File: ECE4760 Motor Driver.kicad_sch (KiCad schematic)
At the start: 29 parts, among them J1 IO, J101 Alternative Motor, J2 Motor / Power, J3 UART, SW1 RESET, U1 STM32G473CETx, U13 AP63205WU, U6 AP7361C-33FGE, U9 MAX13433EETD, X1 48MHz

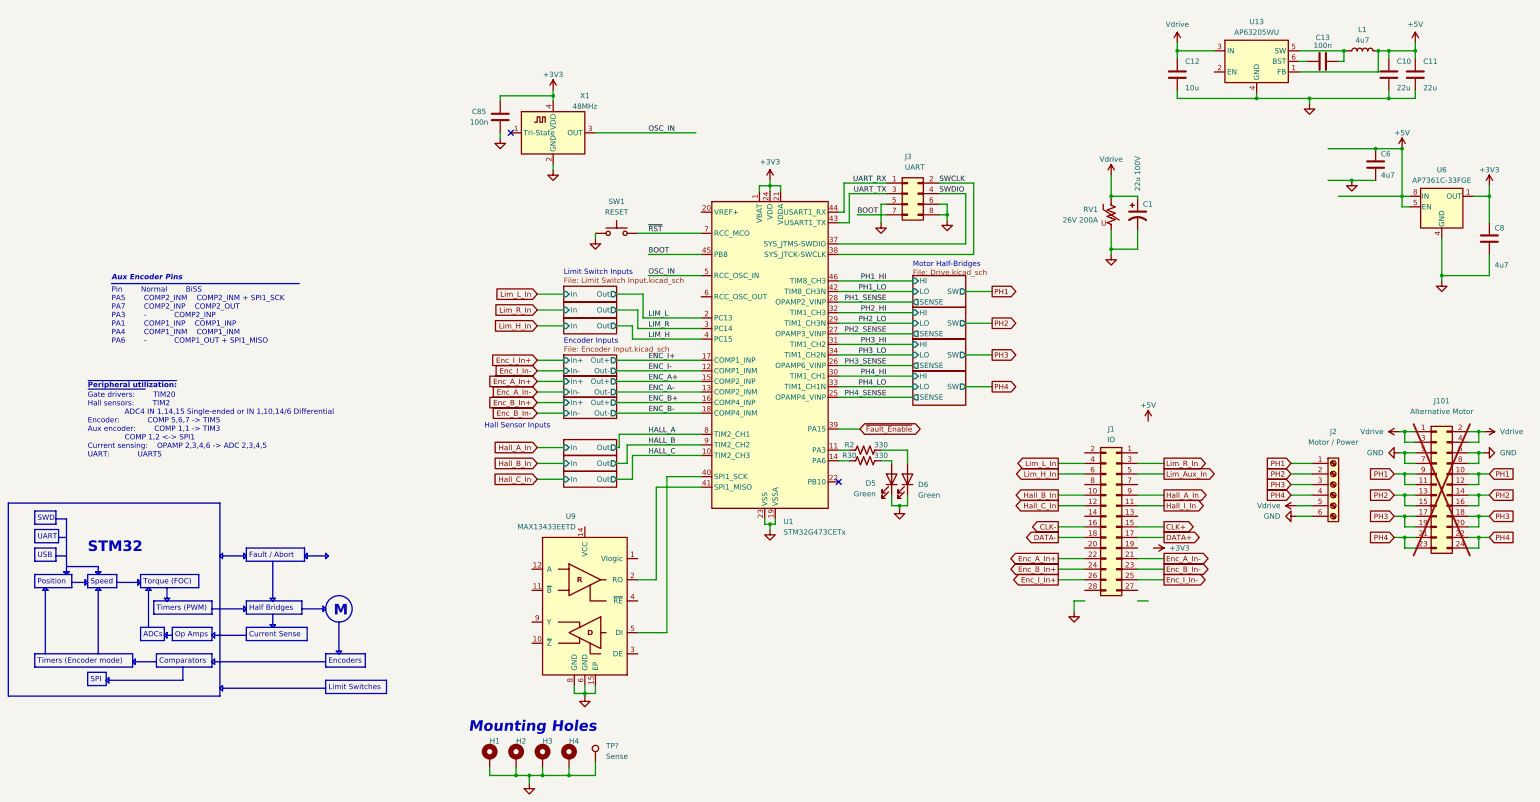
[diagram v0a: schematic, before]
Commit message: Boards ordered!
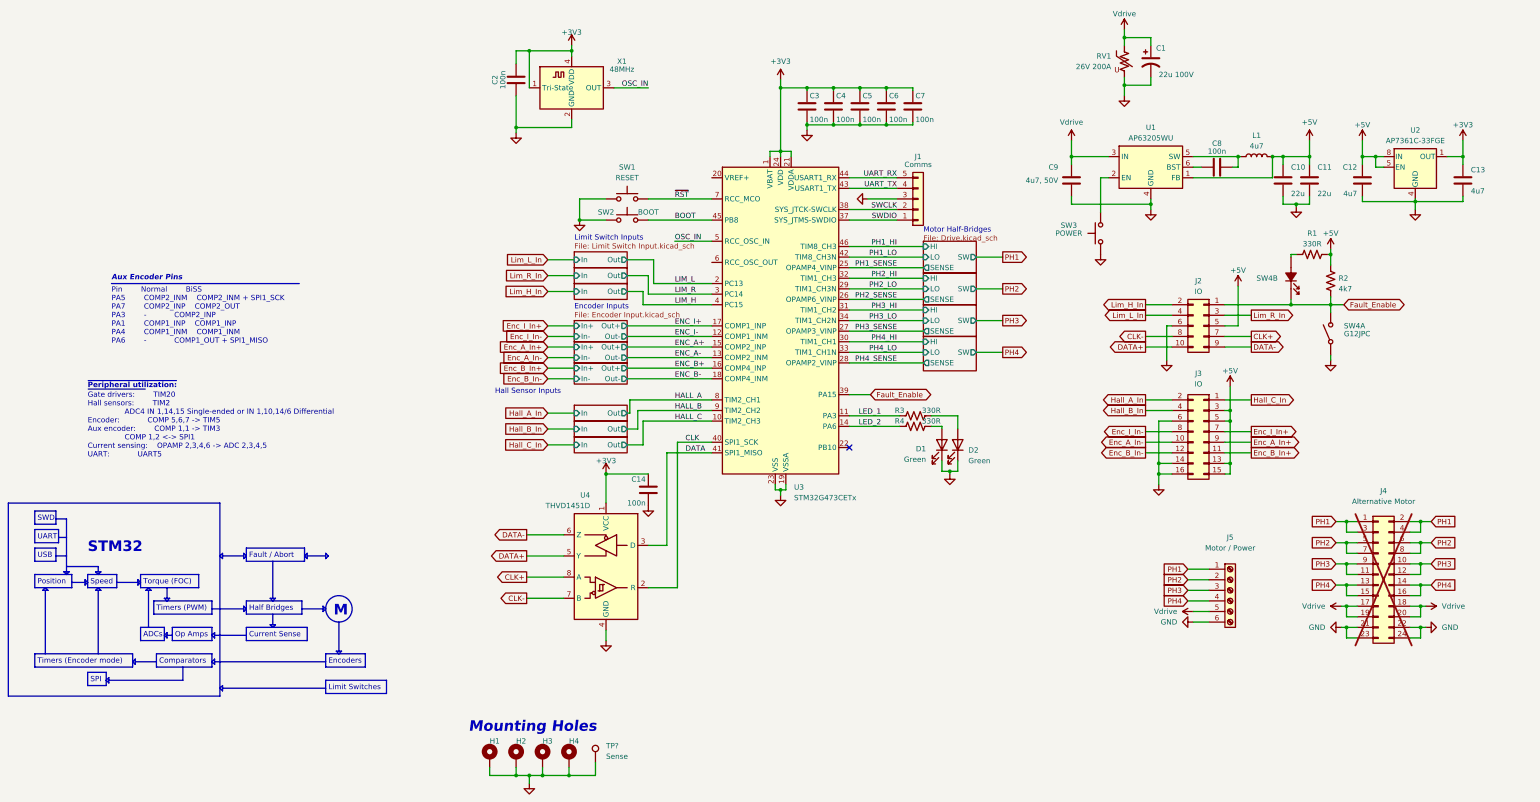
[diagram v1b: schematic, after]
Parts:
- removed J3: UART, Connector_PinHeader_2.54mm:PinHeader_2x04_P2.54mm_Vertical, symbol Connector_Generic:Conn_02x04_Odd_Even
- removed U9: MAX13433EETD, Package_DFN_QFN:DFN-14-1EP_3x3mm_P0.4mm_EP1.78x2.35mm, symbol Interface_UART:MAX13433EETD
- added C14, C3, C4, C5, C6, C7: 100n, Capacitor_SMD:C_0402_1005Metric, symbol Device:C
- added J1: Comms, Connector_PinHeader_2.54mm:PinHeader_1x05_P2.54mm_Vertical, symbol Connector_Generic:Conn_01x05
- added J3: IO, Connector_PinSocket_2.54mm:PinSocket_2x08_P2.54mm_Vertical, symbol Connector_Generic:Conn_02x08_Odd_Even
- added R1: 330R, Resistor_SMD:R_0402_1005Metric, symbol Device:R_US
- added R2: 4k7, Resistor_SMD:R_0402_1005Metric, symbol Device:R_US
- added SW2: BOOT, Button_Switch_SMD:SW_SPST_PTS810, symbol Switch:SW_Push
- added SW3: POWER, Button_Switch_SMD:SW_SPST_PTS810, symbol Switch:SW_Push
- added SW4: G12JPC, Button_Switch_THT:SW_NKK_G1xJP, symbol Switch:SW_SPST_LED
- added U4: THVD1451D, Package_SO:SOIC-8_3.9x4.9mm_P1.27mm, symbol Interface_UART:THVD1451D
- C1: footprint Capacitor_THT:CP_Radial_D6.3mm_P2.50mm -> Capacitor_THT:CP_Radial_D5.0mm_P2.50mm; DigiKey (none) -> P5190-ND; LCSC C7471882 -> (none)
- C10, C11: LCSC (none) -> C86816
- C12: renamed from C6; DigiKey 490-GRM188Z71C475KE21DCT-ND -> (none); LCSC C389010 -> C437557
- C13: renamed from C8; DigiKey 490-GRM188Z71C475KE21DCT-ND -> (none); LCSC C389010 -> C437557
- C8: renamed from C13; DigiKey (none) -> 490-3261-1-ND; LCSC (none) -> C71629
- C9: renamed from C12; value 10u -> 4u7, 50V; LCSC (none) -> C437557
- D1: renamed from D5; footprint LED_SMD:LED_1206_3216Metric -> LED_SMD:LED_0603_1608Metric; DigiKey 160-2018-1-ND -> (none); LCSC C364563 -> C125101
- D2: renamed from D6; footprint LED_SMD:LED_1206_3216Metric -> LED_SMD:LED_0603_1608Metric; DigiKey 160-2018-1-ND -> (none); LCSC C364563 -> C125101
- J2: renamed from J1; footprint Connector_PinSocket_2.54mm:PinSocket_2x14_P2.54mm_Vertical -> Connector_PinSocket_2.54mm:PinSocket_2x05_P2.54mm_Vertical; symbol Connector_Generic:Conn_02x14_Odd_Even -> Connector_Generic:Conn_02x05_Odd_Even
- L1: DigiKey (none) -> 490-5116-1-ND; LCSC (none) -> C82314
- R3: renamed from R2; value 330 -> 330R; LCSC C138006 -> C105875
- R4: renamed from R30; value 330 -> 330R; LCSC C138006 -> C105875
- RV1: footprint Capacitor_SMD:C_1210_3225Metric -> Capacitor_SMD:C_0603_1608Metric; Comments (none) -> Reduced size for LCSC stock -- reccomend increasing to larg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; DigiKey F3823CT-ND -> (none); LCSC C2659457 -> C2655584
- U1: renamed from U13; LCSC (none) -> C2071056
- U2: renamed from U6; footprint Package_DFN_QFN:DFN-8-1EP_3x3mm_P0.5mm_EP1.65x2.38mm -> Package_DFN_QFN:DFN-8-1EP_3x3mm_P0.65mm_EP1.55x2.4mm
- U3: renamed from U1; LCSC (none) -> C730111
- X1: LCSC C3034286 -> C390534
- renumbered C85 to C2, J101 to J4, J2 to J5
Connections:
- net Lim_Aux_In is gone; now on net +5V: J2.5 (Pin_5)
- net ~{Fault_Enable} is gone; now on net Fault_Enable: U3.39 (PA15)
- net +3V3: now also X1.1 (Tri-State), C14.1, C3.1, C4.1, C5.1, C6.1, C7.1, U4.1 (VCC)
- net +5V: now also J3.13 (Pin_13), J3.15 (Pin_15), J3.3 (Pin_3), J3.5 (Pin_5), R1.2, R2.1
- net BOOT: now also SW2.2
- net CLK+: now also J2.7 (Pin_7), U4.8 (A); no longer J2.15 (Pin_15)
- net CLK-: now also J2.8 (Pin_8), U4.7 (B); no longer J2.16 (Pin_16)
- net DATA+: now also J2.10 (Pin_10), U4.5 (Y); no longer J2.17 (Pin_17)
- net DATA-: now also J2.9 (Pin_9), U4.6 (Z); no longer J2.18 (Pin_18)
- net Enc_A_In+: now also J3.9 (Pin_9); no longer J2.22 (Pin_22)
- net Enc_A_In-: now also J3.10 (Pin_10); no longer J2.21 (Pin_21)
- net Enc_B_In+: now also J3.11 (Pin_11); no longer J2.24 (Pin_24)
- net Enc_B_In-: now also J3.12 (Pin_12); no longer J2.23 (Pin_23)
- net Enc_I_In+: now also J3.7 (Pin_7); no longer J2.26 (Pin_26)
- net Enc_I_In-: now also J3.8 (Pin_8); no longer J2.25 (Pin_25)
- net GND: now also J2.6 (Pin_6), J4.21 (Pin_21), J4.22 (Pin_22), J4.23 (Pin_23), J4.24 (Pin_24), C14.2, C3.2, C4.2, C5.2, C6.2, C7.2, J1.3 (Pin_3), J3.14 (Pin_14), J3.16 (Pin_16), J3.6 (Pin_6), SW2.1, SW3.1, SW4.2 (COM), U4.4 (GND); no longer J4.5 (Pin_5), J4.6 (Pin_6), J4.7 (Pin_7), J4.8 (Pin_8)
- net Hall_A_In: now also J3.2 (Pin_2); no longer J2.9 (Pin_9)
- net Hall_B_In: now also J3.4 (Pin_4); no longer J2.10 (Pin_10)
- net Hall_C_In: now also J3.1 (Pin_1); no longer J2.12 (Pin_12)
- net Lim_H_In: now also J2.2 (Pin_2); no longer J2.6 (Pin_6)
- net PH1: now also J4.1 (Pin_1), J4.2 (Pin_2), J4.3 (Pin_3), J4.4 (Pin_4); no longer J4.10 (Pin_10), J4.11 (Pin_11), J4.12 (Pin_12), J4.9 (Pin_9)
- net PH1_SENSE: now also U3.25 (PB11); no longer U3.28 (PB14)
- net PH2: now also J4.5 (Pin_5), J4.6 (Pin_6), J4.7 (Pin_7), J4.8 (Pin_8); no longer J4.13 (Pin_13), J4.14 (Pin_14), J4.15 (Pin_15), J4.16 (Pin_16)
- net PH2_SENSE: now also U3.26 (PB12); no longer U3.27 (PB13)
- net PH3: now also J4.10 (Pin_10), J4.11 (Pin_11), J4.12 (Pin_12), J4.9 (Pin_9); no longer J4.17 (Pin_17), J4.18 (Pin_18), J4.19 (Pin_19), J4.20 (Pin_20)
- net PH3_SENSE: now also U3.27 (PB13); no longer U3.26 (PB12)
- net PH4: now also J4.13 (Pin_13), J4.14 (Pin_14), J4.15 (Pin_15), J4.16 (Pin_16); no longer J4.21 (Pin_21), J4.22 (Pin_22), J4.23 (Pin_23), J4.24 (Pin_24)
- net PH4_SENSE: now also U3.28 (PB14); no longer U3.25 (PB11)
- net SWCLK: now also J1.2 (Pin_2)
- net SWDIO: now also J1.1 (Pin_1)
- net UART_RX: now also J1.5 (Pin_5)
- net UART_TX: now also J1.4 (Pin_4)
- net Vdrive: now also J4.17 (Pin_17), J4.18 (Pin_18), J4.19 (Pin_19), J4.20 (Pin_20); no longer J4.1 (Pin_1), J4.2 (Pin_2), J4.3 (Pin_3), J4.4 (Pin_4)
- net LED_2: now reaches R4.1, U3.14 (PA6)
- net at U1.2 (EN): now also SW3.2
- net LED_1: now reaches R3.1, U3.11 (PA3)
- net DATA: now reaches U3.41 (PB4)
- net DATA: now also U4.3 (D)
- net CLK: now reaches U3.40 (PB3)
- net CLK: now also U4.2 (R)
- net Fault_Enable: now reaches J2.1 (Pin_1)
- net Fault_Enable: now also R2.2, SW4.3, SW4.6 (K)
- removed net Hall_I_In: J2.11 (Pin_11)
- new net: R1.1, SW4.5 (A)
- no-connect marks 2 -> 1
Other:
- moved on the sheet: C1, C10, C11, C12, C13, C2, C8, C9, D1, D2, J4, J5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
